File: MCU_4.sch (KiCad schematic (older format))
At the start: 18 parts, among them U2 STM32F051K6Ux

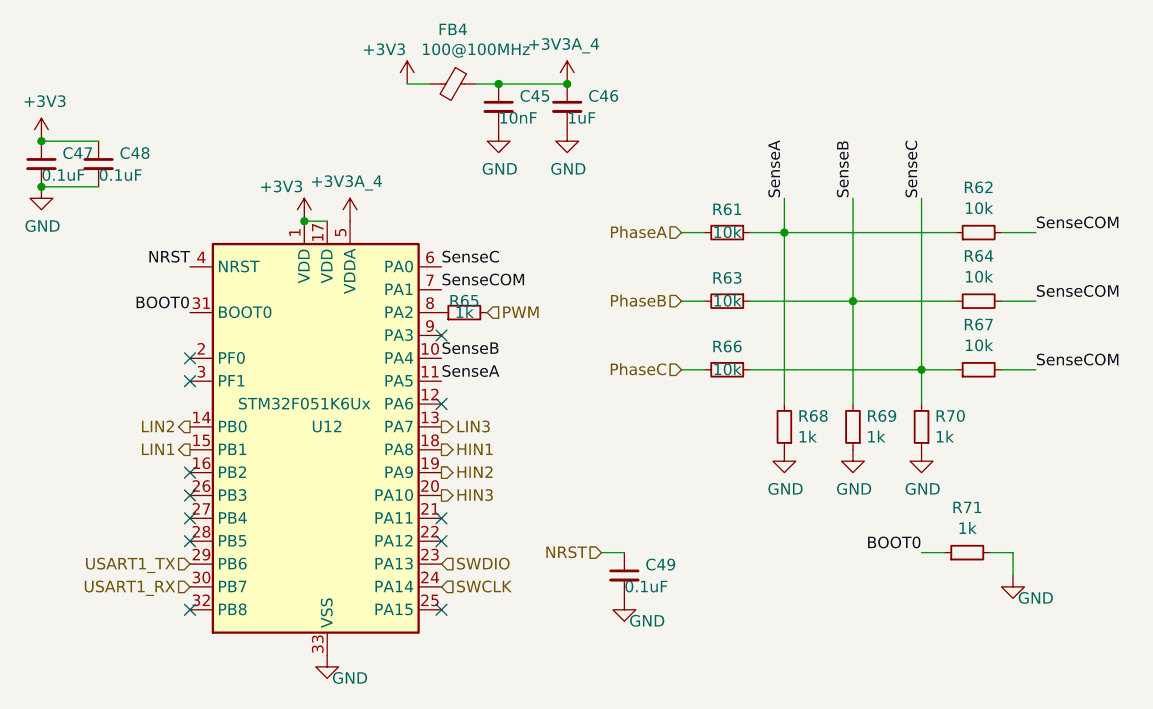
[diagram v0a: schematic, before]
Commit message: Added stuff
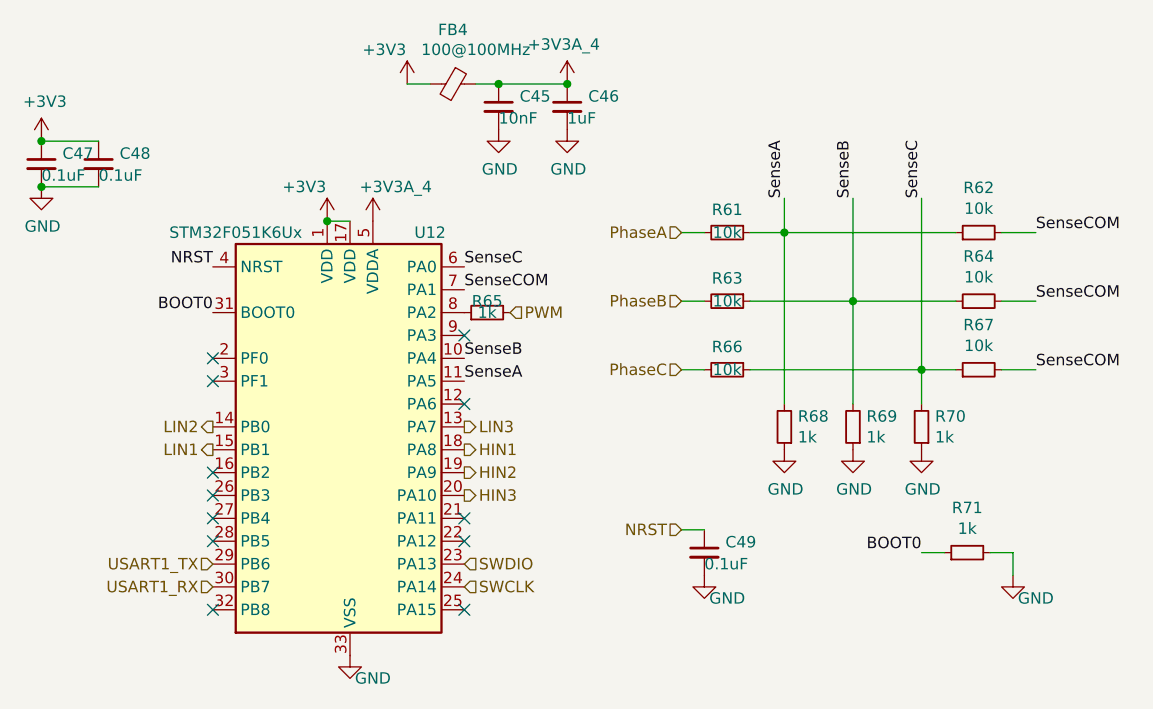
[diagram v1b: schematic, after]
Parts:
- removed R24: 1k, Resistor_SMD:R_0402_1005Metric, symbol Device:R_Small
- removed U2: STM32F051K6Ux, Package_DFN_QFN:QFN-32-1EP_5x5mm_P0.5mm_EP3.45x3.45mm, symbol MCU_ST_STM32F0:STM32F051K6Ux
- added R65: 1k, Resistor_SMD:R_0402_1005Metric, symbol Device:R_Small
- added U12: STM32F051K6Ux, Package_DFN_QFN:QFN-32-1EP_5x5mm_P0.5mm_EP3.45x3.45mm, symbol MCU_ST_STM32F0:STM32F051K6Ux
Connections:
- net +3.3VA_4: now also U12.5 (VDDA)
- net +3V3: now also U12.1 (VDD), U12.17 (VDD)
- net BOOT0: now also U12.31 (BOOT0)
- net GND: now also U12.33 (VSS)
- net HIN1: now also U12.18 (PA8)
- net HIN2: now also U12.19 (PA9)
- net HIN3: now also U12.20 (PA10)
- net LIN1: now also U12.15 (PB1)
- net LIN2: now also U12.14 (PB0)
- net LIN3: now also U12.13 (PA7)
- net NRST: now also U12.4 (NRST)
- net PWM: now also R65.2
- net SWCLK: now also U12.24 (PA14)
- net SWDIO: now also U12.23 (PA13)
- net SenseA: now also U12.11 (PA5)
- net SenseB: now also U12.10 (PA4)
- net SenseC: now also U12.6 (PA0)
- net SenseCOM: now also U12.7 (PA1)
- net USART1_RX: now also U12.30 (PB7)
- net USART1_TX: now also U12.29 (PB6)
- new net: R65.1, U12.8 (PA2)
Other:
- moved on the sheet: C49
